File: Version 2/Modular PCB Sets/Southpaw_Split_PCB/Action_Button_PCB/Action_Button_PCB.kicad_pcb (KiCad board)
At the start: 2 copper layers, 150 x 107 mm, 28 parts, among them J1 Conn_01x06_Socket, J2 Conn_01x07_Socket, J3 Conn_01x07_Socket, X1 SW_SPST, Y1 SW_SPST

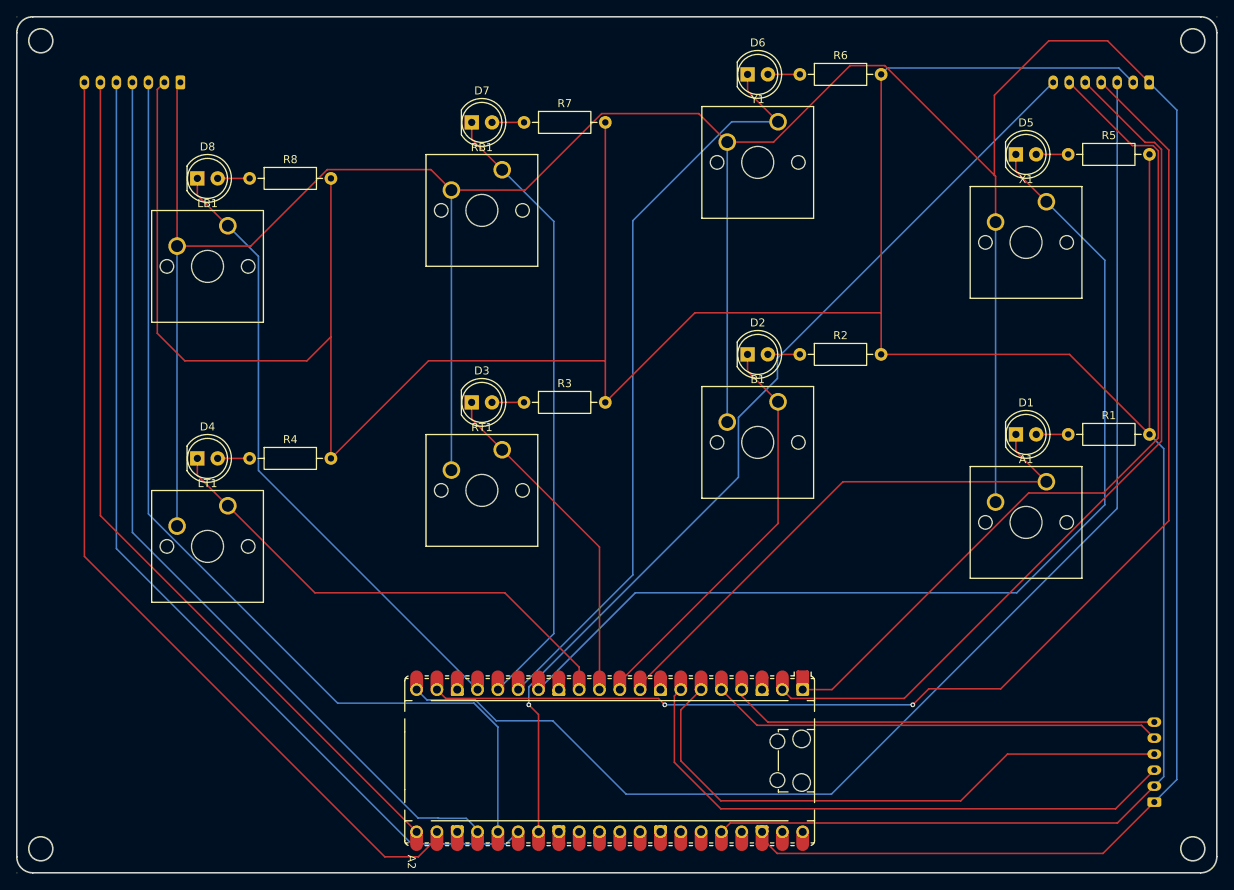
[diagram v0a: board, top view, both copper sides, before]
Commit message: Finalized design and uploaded gerbers to JLCpcb, waiting for boards to come in
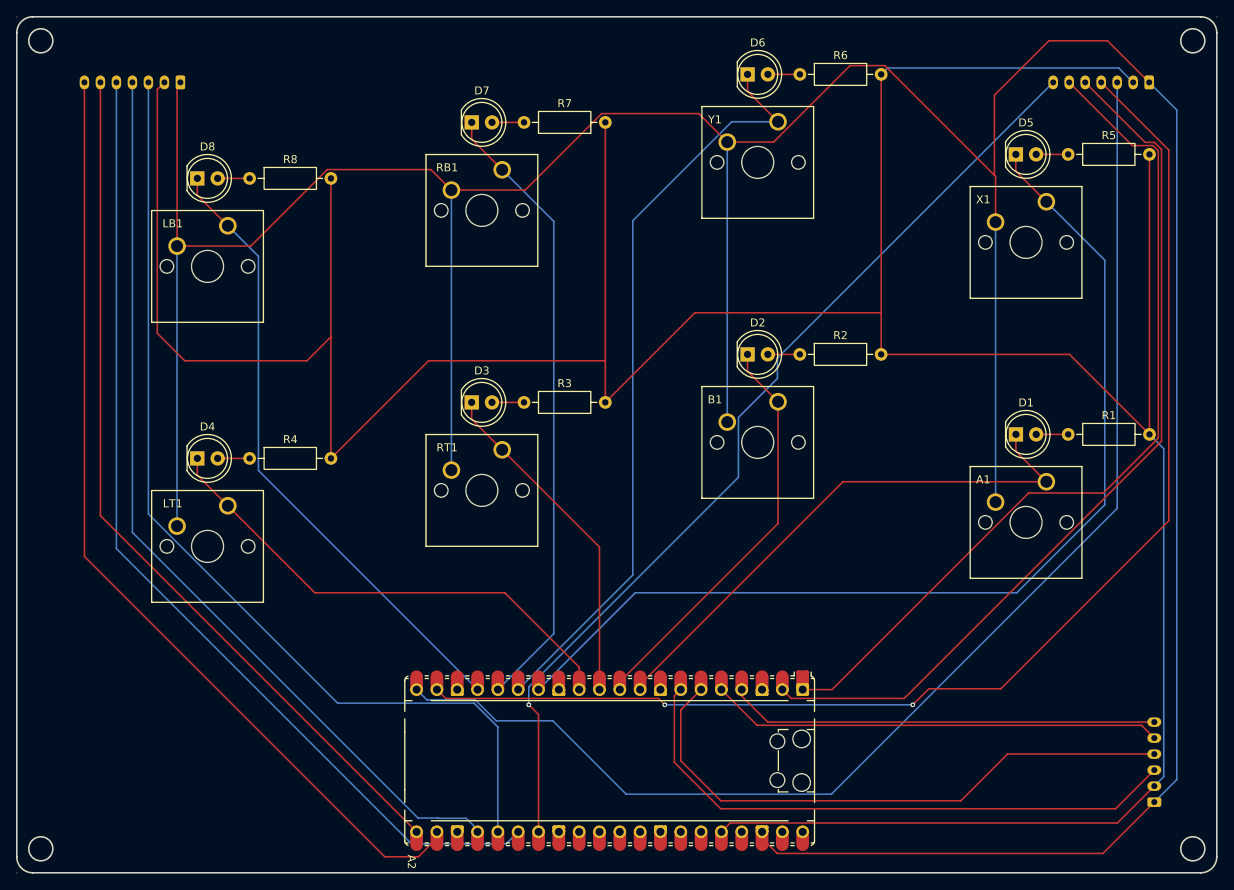
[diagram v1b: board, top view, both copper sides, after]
